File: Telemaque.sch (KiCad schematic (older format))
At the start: 75 parts, among them J1 Test, J2 Test, J3 Test, J4 Test, J5 Conn_01x01, J6 Conn_01x01, J7 Conn_01x01, P1 CONN_01X03, P2 CONN_01X10, P3 SMA, P4 CONN_01X05, P5 SMA, U1 LMC6482, U2 LD1117STR, U3 LD1117S50TR, U4 ACS723LLCTR-40AU-T, U5 LD1117S50TR, U6 LMC6482

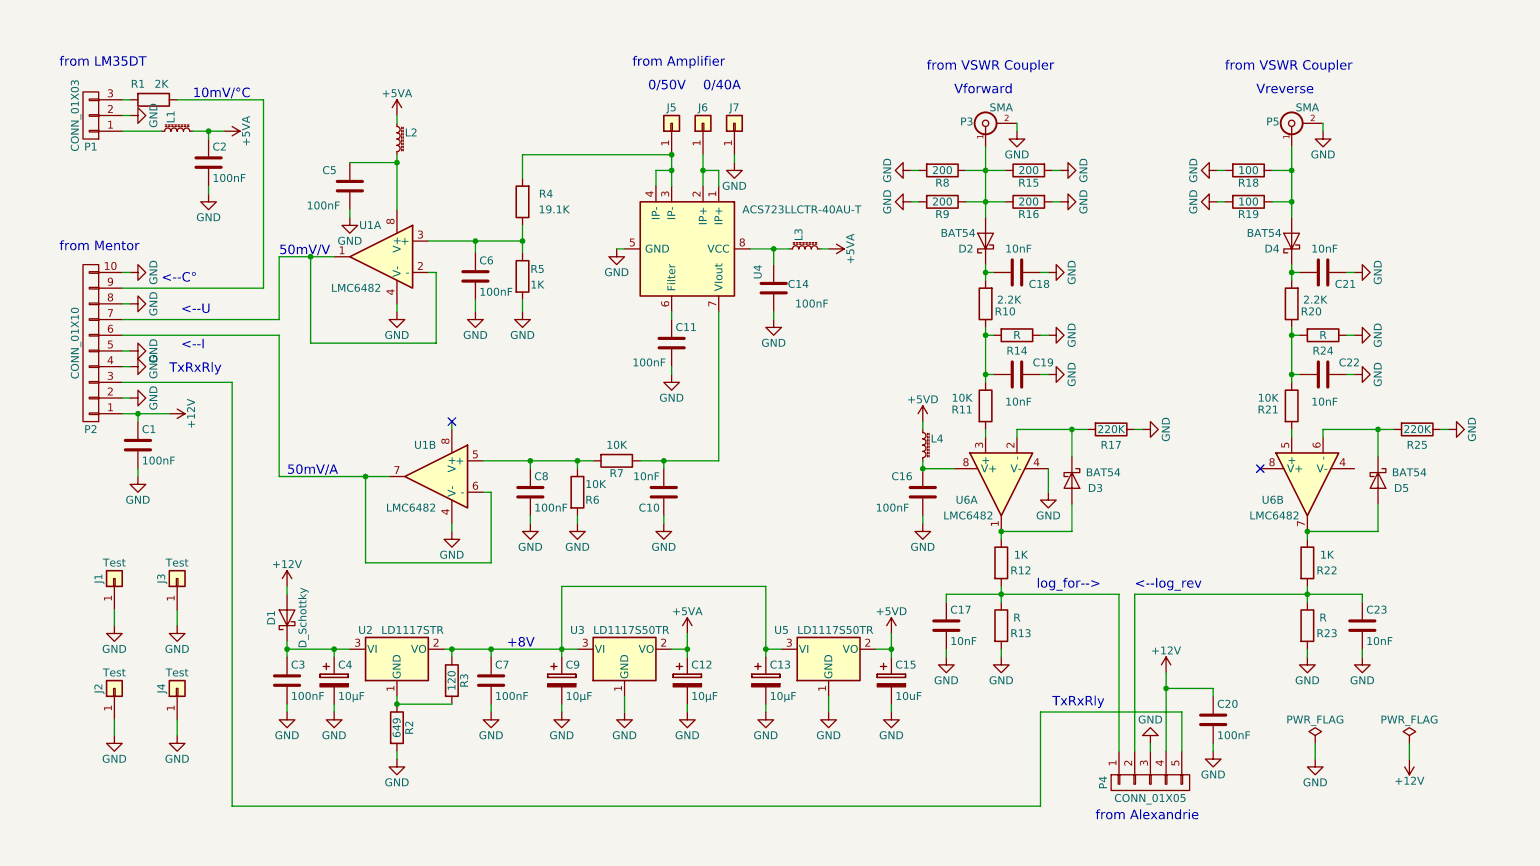
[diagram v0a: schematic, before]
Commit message: Add files via upload
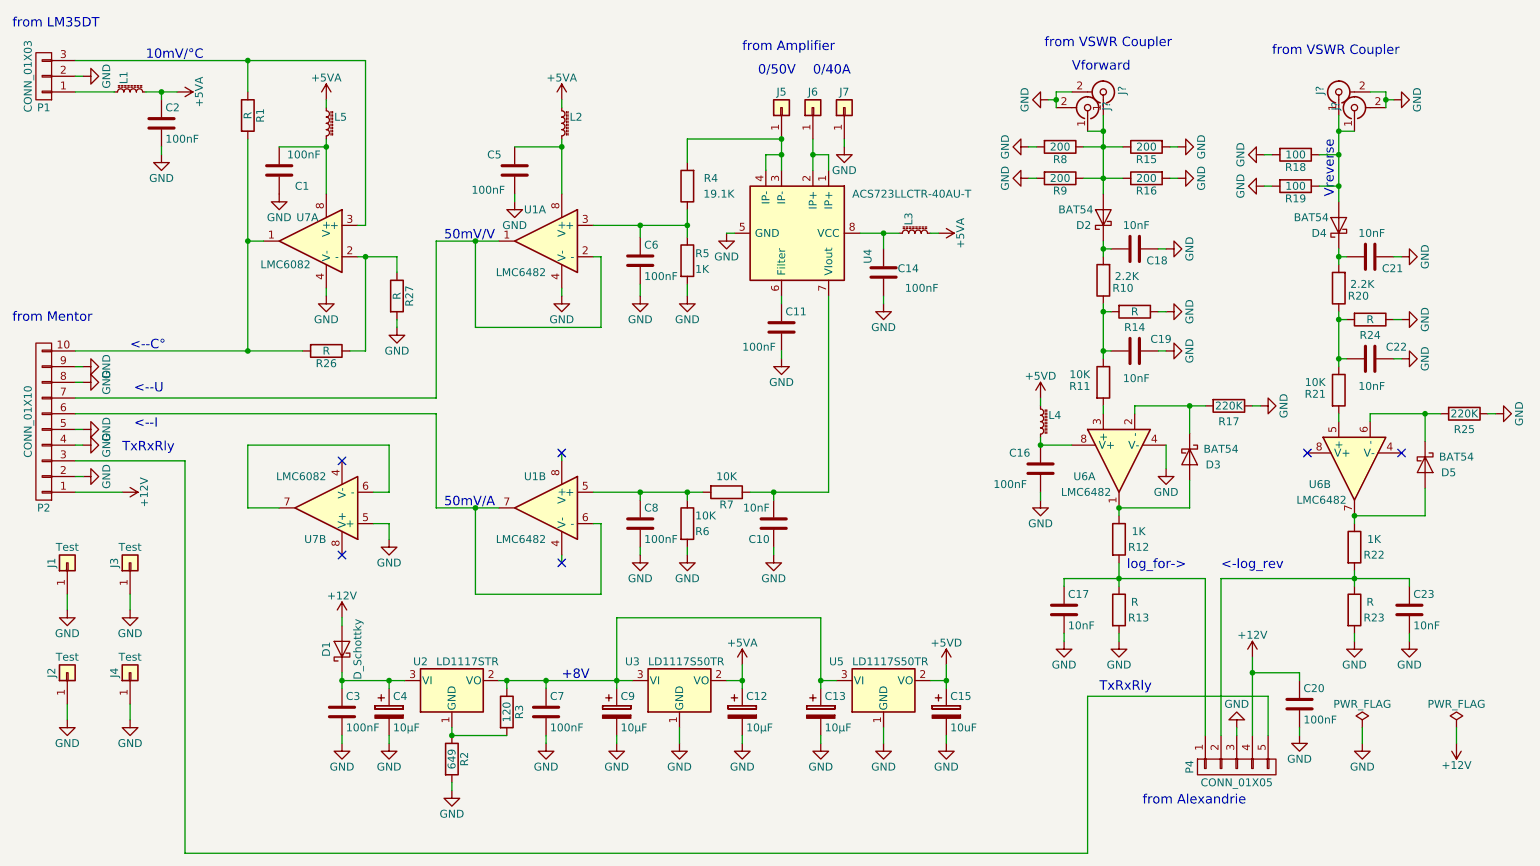
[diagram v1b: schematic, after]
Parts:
- removed P3, P5: SMA, SMA_PINS:SMA_PINS, symbol BNC
- added J? (x4): Conn_Coaxial, symbol Conn_Coaxial
- added L5: L_Core_Ferrite_Small, Inductors_SMD:L_0805_HandSoldering, symbol L_Core_Ferrite_Small
- added R26, R27: R, Resistors_SMD:R_0805_HandSoldering, symbol R
- added U7: LMC6082, Housings_SOIC:SO-8_5.3x6.2mm_Pitch1.27mm, symbol LMC6082
- C10, C17, C18, C19, C21, C22, C23: footprint Capacitors_SMD:C_0805_HandSoldering -> Resistors_SMD:R_0805_HandSoldering
- C6, C8: footprint Capacitors_SMD:C_0805_HandSoldering -> Capacitors_SMD:C_1206_HandSoldering
- J5, J6, J7: footprint Conn_Wurth:Redcube_100A_M3_V -> Conn_Wurth:Wurth
- R1: value 2K -> R
- U4: footprint Housings_SOIC:SOIC-8_3.9x4.9mm_Pitch1.27mm -> Housings_SOIC:SO-8_5.3x6.2mm_Pitch1.27mm
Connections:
- net +12V: no longer C1.1
- net +5VA: now also L5.1
- net GND: now also P2.9 (P9), J?.2 (Ext), J?.2 (Ext), J?.2 (Ext), J?.2 (Ext), R27.2, U7.4 (V-), U7.5 (+); no longer P2.10 (P10), U1.4 (V-)
- net at R1.1: now also P1.3 (P3), U7.3 (+); no longer P2.9 (P9)
- net at R1.2: now also P2.10 (P10), R26.2, U7.1; no longer P1.3 (P3)
- net at D4.2 (A), R18.1, R19.1: now also J?.1 (In), J?.1 (In)
- net at D2.2 (A), R15.1, R16.1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: now also J?.1 (In), J?.1 (In)
- new net: R26.1, R27.1, U7.2 (-)
- new net: C1.1, L5.2, U7.8 (V+)
- new net: U7.6 (-), U7.7
- no-connect marks 2 -> 6
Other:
- note added: "<-log_rev"
- note added: "log_for->"
- note removed: "<--log_rev"
- note removed: "log_for-->"
- moved on the sheet: C10, C11, C12, C13, C14, C15, C16, C17, C18, C19, C2, C20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

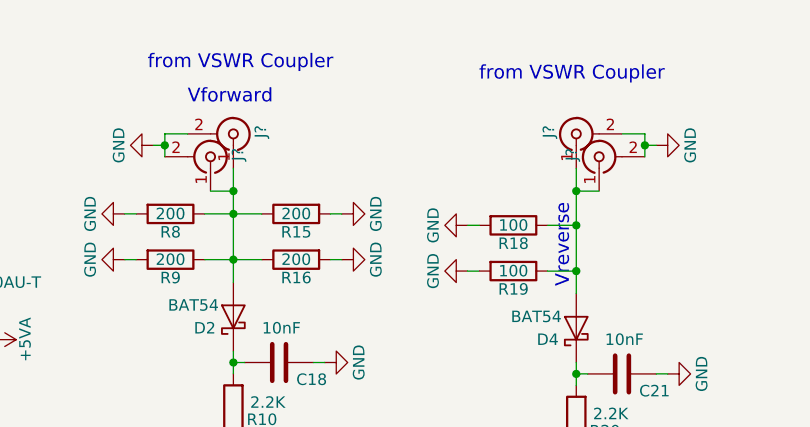
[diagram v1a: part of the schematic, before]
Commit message: Add files via upload
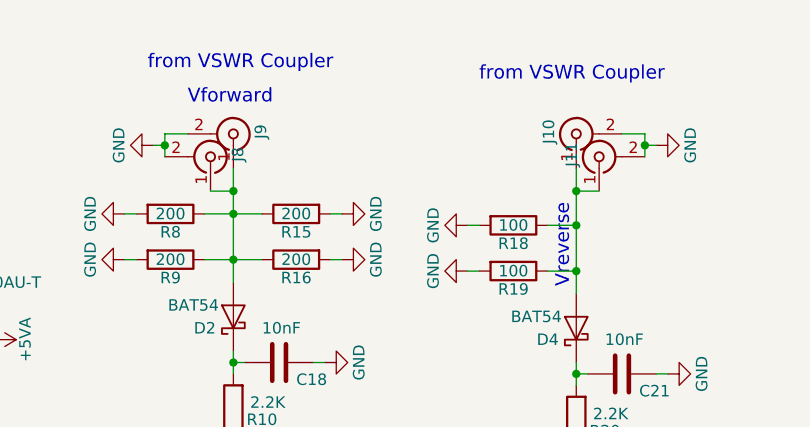
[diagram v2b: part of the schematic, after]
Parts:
- gave numbers to parts that had none: 4
